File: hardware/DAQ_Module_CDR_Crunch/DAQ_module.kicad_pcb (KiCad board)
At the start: 4 copper layers, 38 x 58.5 mm, 56 parts, among them J1 Conn_01x10_Pin, J3 Conn_01x20_Pin, U1 MCP3564RT-E/ST, U2 MAX31855KASA, U3 MAX31855KASA, U5 TPS70933DBVR, U6 TPS70933DBVR, U7 TPS70933DBVR, U8 MAX31855KASA

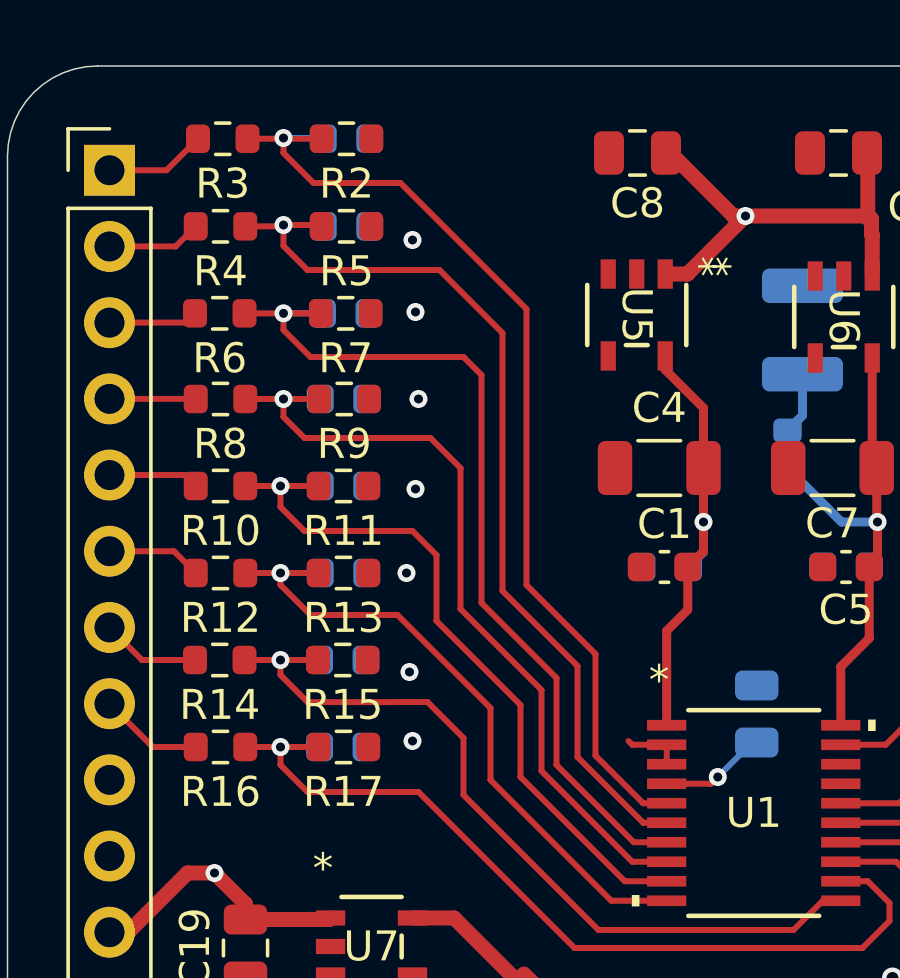
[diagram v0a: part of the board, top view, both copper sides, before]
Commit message: Finished PCBs
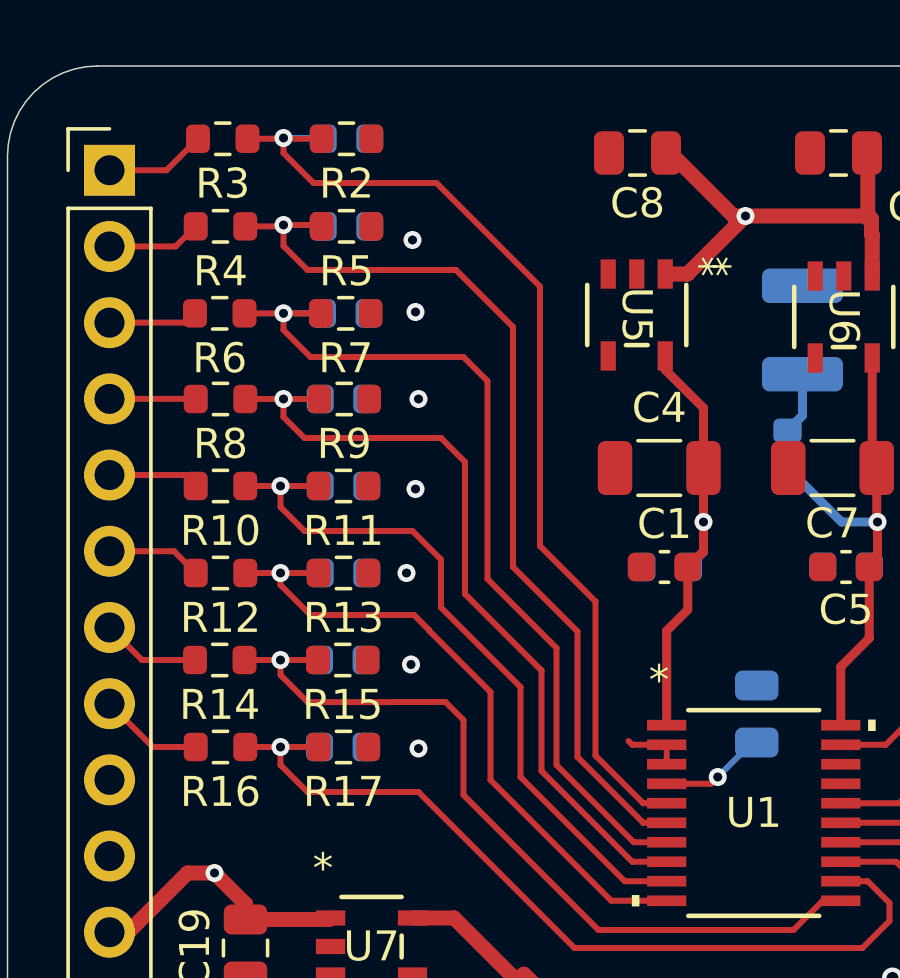
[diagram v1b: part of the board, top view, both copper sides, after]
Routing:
- net /ADC_AI_Filt_0: track 33.5 -> 34.2 mm
